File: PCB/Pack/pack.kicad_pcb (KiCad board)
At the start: 2 copper layers, 100 x 100 mm, 76 parts, among them J1 Conn_01x01, J2 Conn_01x01, J3 Conn_01x01, J4 Conn_01x01, J5 Conn_01x01, J6 Conn_01x01, J7 Conn_01x02, J8 Conn_01x02

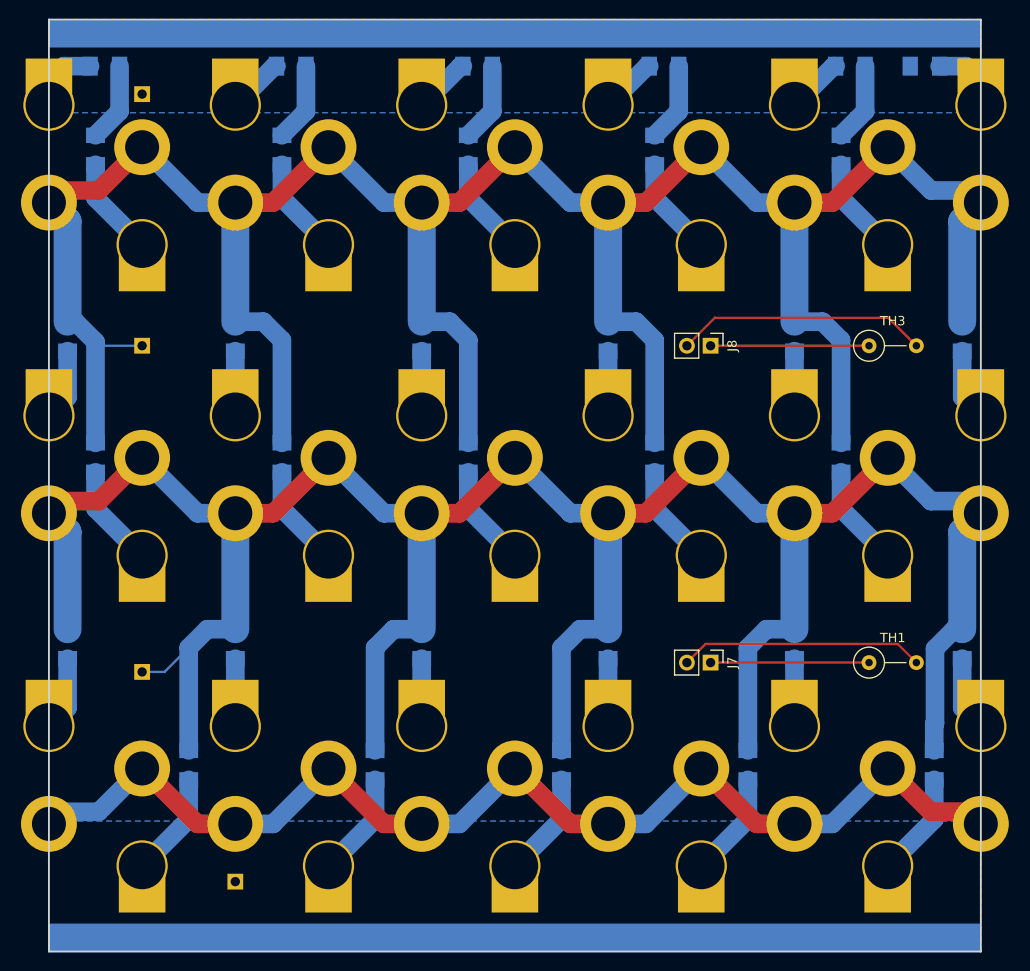
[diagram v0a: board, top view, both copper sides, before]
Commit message: minor stuff
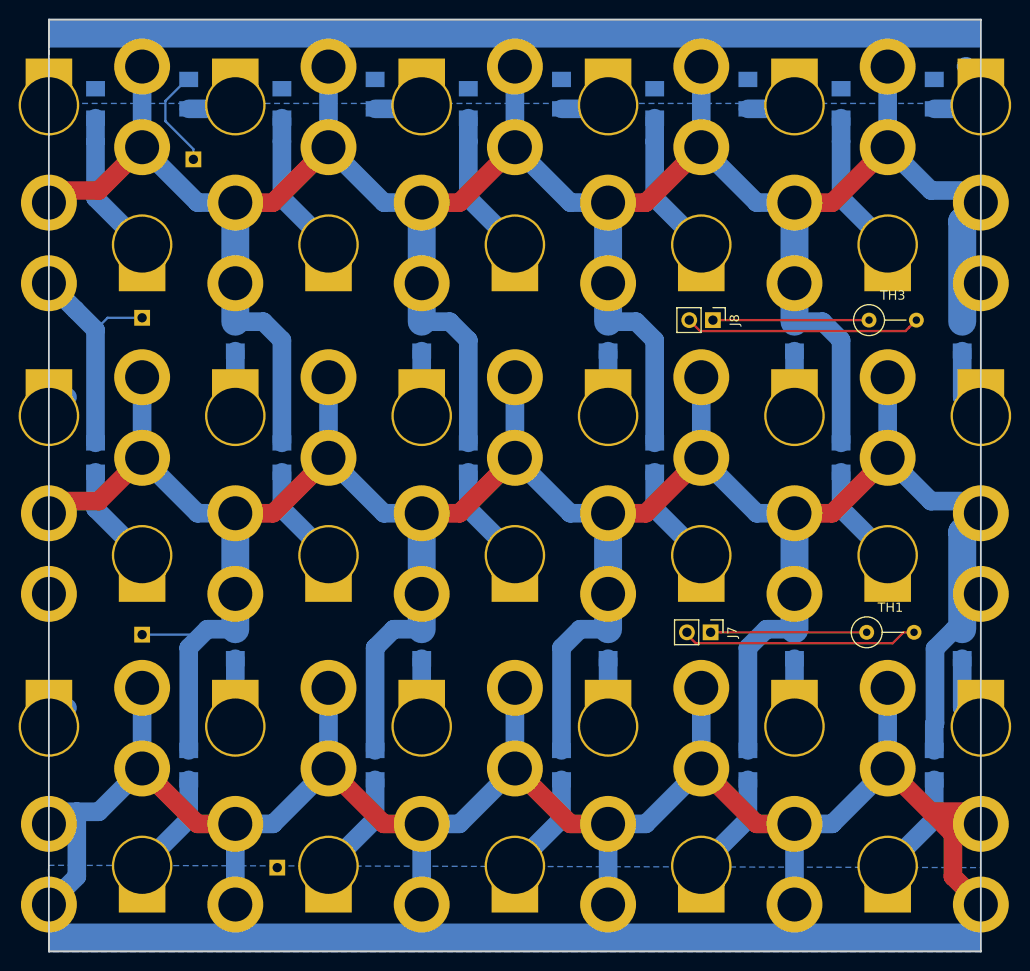
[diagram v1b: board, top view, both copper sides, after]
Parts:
- removed F1, F2, F3: Fuse, Fuse_Holders_and_Fuses:Fuse_SMD1206_Wave
- moved F13 11.4 mm to (35.0, 8.00), turned to 270 degrees
- moved F19 11.4 mm to (55.0, 8.00), turned to 270 degrees
- moved F25 11.4 mm to (75.0, 8.00), turned to 270 degrees
- moved F7 11.4 mm to (15.0, 8.00), turned to 270 degrees
- moved J1 8.90 mm to (15.5, 15.0)
- moved F10 5.00 mm to (25.0, 9.00)
- moved F16 5.00 mm to (45.0, 9.00)
- moved F22 5.00 mm to (65.0, 9.00)
- moved F28 5.00 mm to (85.0, 9.00)
- moved F4 5.00 mm to (5.00, 9.00)
- moved J4 4.74 mm to (24.5, 91.0)
- moved J3 4.00 mm to (10.0, 66.0)
- moved TH1 3.26 mm to (87.8, 65.8)
- moved J7 3.25 mm to (71.0, 65.8)
- moved F31 3.16 mm to (95.0, 8.00), turned to 270 degrees
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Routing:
- net Net-(BT12-Pad2): track 120.9 -> 218.5 mm
- net Net-(BT1-Pad2): track 281.5 -> 320.5 mm
- net Net-(BT11-Pad2): track 280.4 -> 316.8 mm
- net Net-(F1-Pad1): track 42.4 -> 11.0 mm
- net Net-(BT7-Pad1): track 10.6 -> 16.7 mm
- net Net-(BT33-Pad1): track 6.26 -> 0.99 mm
- net Net-(BT25-Pad1): track 10.6 -> 15.6 mm
- net Net-(BT19-Pad1): track 10.6 -> 15.6 mm
- net Net-(BT13-Pad1): track 10.6 -> 15.6 mm
- net Net-(BT1-Pad1): track 10.6 -> 15.6 mm
- net Net-(BT32-Pad1): track 5.93 -> 0.99 mm
- net Net-(BT31-Pad1): track 3.24 -> 0.00 mm
- net Net-(J8-Pad2): track 27.1 -> 25.3 mm
- net Net-(BT22-Pad1): track 6.15 -> 5.16 mm
- net Net-(BT16-Pad1): track 6.15 -> 5.16 mm
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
